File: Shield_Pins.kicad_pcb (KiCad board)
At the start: 2 copper layers, 76 x 38.3 mm, 40 parts, among them J1 Conn_01x04_Male, J11 Screw_Terminal_01x02, J12 DB9_Male, J2 Conn_01x06_Male, J3 Conn_01x06_Male, J4 Conn_01x04_Male, J5 Conn_01x01_Male, J6 Conn_01x06_Male, J7 Conn_01x15_Male, J8 Conn_01x15_Male, J9 Conn_01x02_Male, SW1 SW_SPDT, U1 MCP2515-xSO, U2 MCP2551-I-SN, U3 LD1117S50TR_SOT223, Y1 8MHz Crystal

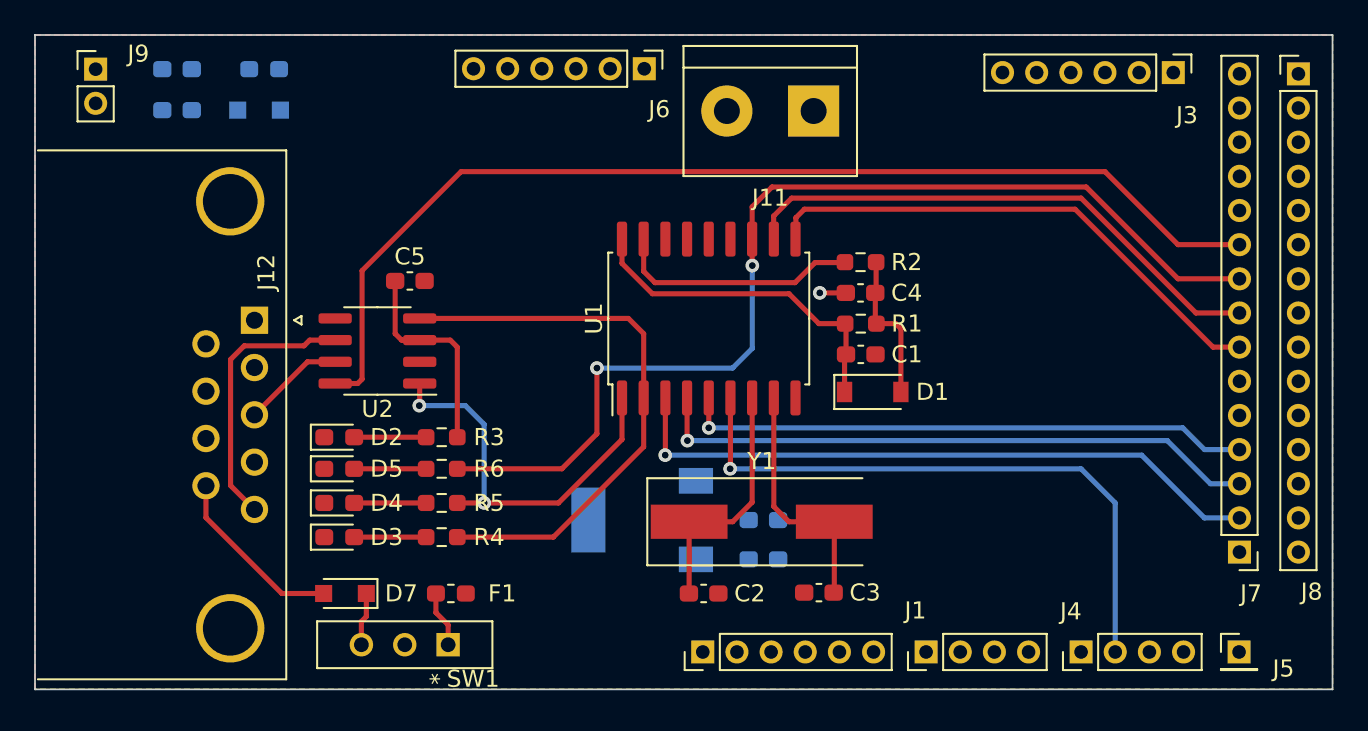
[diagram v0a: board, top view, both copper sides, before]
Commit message: Complete Board (1)
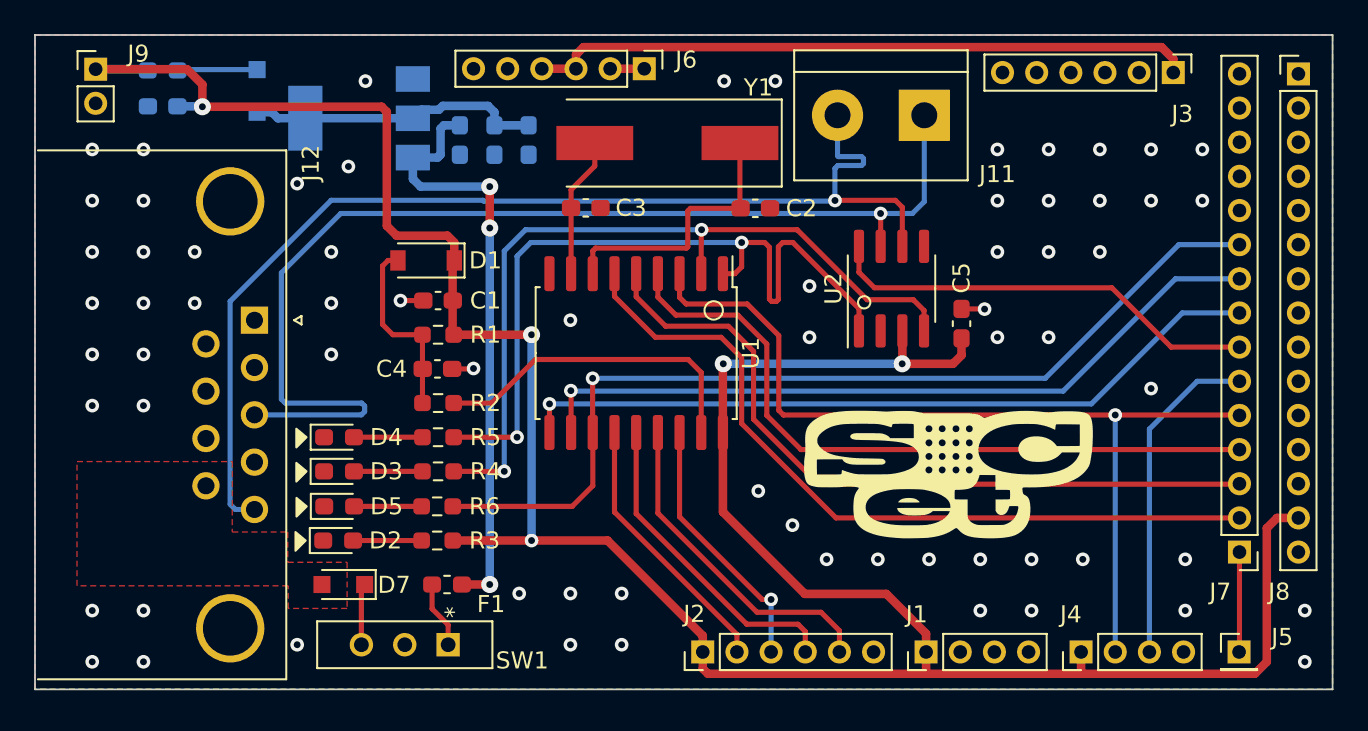
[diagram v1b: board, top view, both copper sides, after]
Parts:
- added G***: LOGO, CANBusShield:SoCET_logo, F.Cu at (143.0, 96.0)
- moved C5 32.4 mm to (143.9, 87.2), turned to 90 degrees
- moved U2 30.3 mm to (139.8, 85.2), turned to 90 degrees
- moved CIN1 30.3 mm to (114.5, 76.5), turned to -90 degrees
- moved U3 28.8 mm to (108.6, 75.2)
- moved D1 27.3 mm to (112.5, 83.5), turned to 180 degrees
- moved C3 26.3 mm to (121.9, 80.4), turned to 0 degrees
- moved COUT1 26.2 mm to (118.5, 76.5), turned to -90 degrees
- moved R2 26.1 mm to (113.2, 91.8), turned to 0 degrees
- moved C4 25.2 mm to (113.2, 89.8), turned to 0 degrees
- moved C1 24.9 mm to (113.2, 85.8), turned to 180 degrees
- moved R1 24.8 mm to (113.2, 87.8), turned to 180 degrees
- moved Y1 22.9 mm to (126.7, 76.6), turned to 180 degrees
- moved C2 22.8 mm to (131.8, 80.5)
- moved C6 18.7 mm to (116.5, 76.5), turned to -90 degrees
- moved J11 6.48 mm to (141.7, 75.0)
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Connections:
- R6 pad 1: IO19 -> IO20
- U1 pad 10: IO17 -> IO18
- U1 pad 11: IO18 -> IO19
- U1 pad 12: IO19 -> IO20
- U1 pad 3: IO8 -> IO11
- U1 pad 4: IO9 -> IO10
- U1 pad 5: IO10 -> IO9
- U1 pad 6: IO11 -> IO8
- U2 pad 8: IO20 -> IO17
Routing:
- net +5V: track 32.5 -> 163.0 mm, vias 0 -> 5
- net CANH: track 6.01 -> 65.6 mm, vias 0 -> 1
- net CANL: track 16.0 -> 65.7 mm, vias 0 -> 1
- net +3.3V: track 0.00 -> 39.1 mm
- net 12V_OBD: track 0.00 -> 35.3 mm, vias 0 -> 3
- net TXCAN: track 23.8 -> 46.5 mm
- net IO12: track 0.00 -> 19.5 mm
- net IO.SDO: track 0.00 -> 19.4 mm
- net IO.SDI: track 0.00 -> 18.7 mm
- net IO19: track 62.0 -> 44.3 mm, vias 2 -> 1
- net 5V_OBD: track 0.00 -> 17.3 mm
- net IO11: track 36.3 -> 53.5 mm
- net IO.SCK: track 0.00 -> 15.8 mm
- net IO.CSB: track 0.00 -> 15.4 mm, vias 0 -> 1
- net RXCAN: track 33.2 -> 46.5 mm, vias 0 -> 2
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- added copper zone on F.Cu, net 12V_OBD_IN
